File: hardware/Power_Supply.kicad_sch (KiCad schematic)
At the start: 66 parts, among them IC1 LM13700, IC2 LM13700, IC3 LM13700, J5 USB_B, SW1 POWER, U1 TL064, U19 TL064, U20 ADUM3160

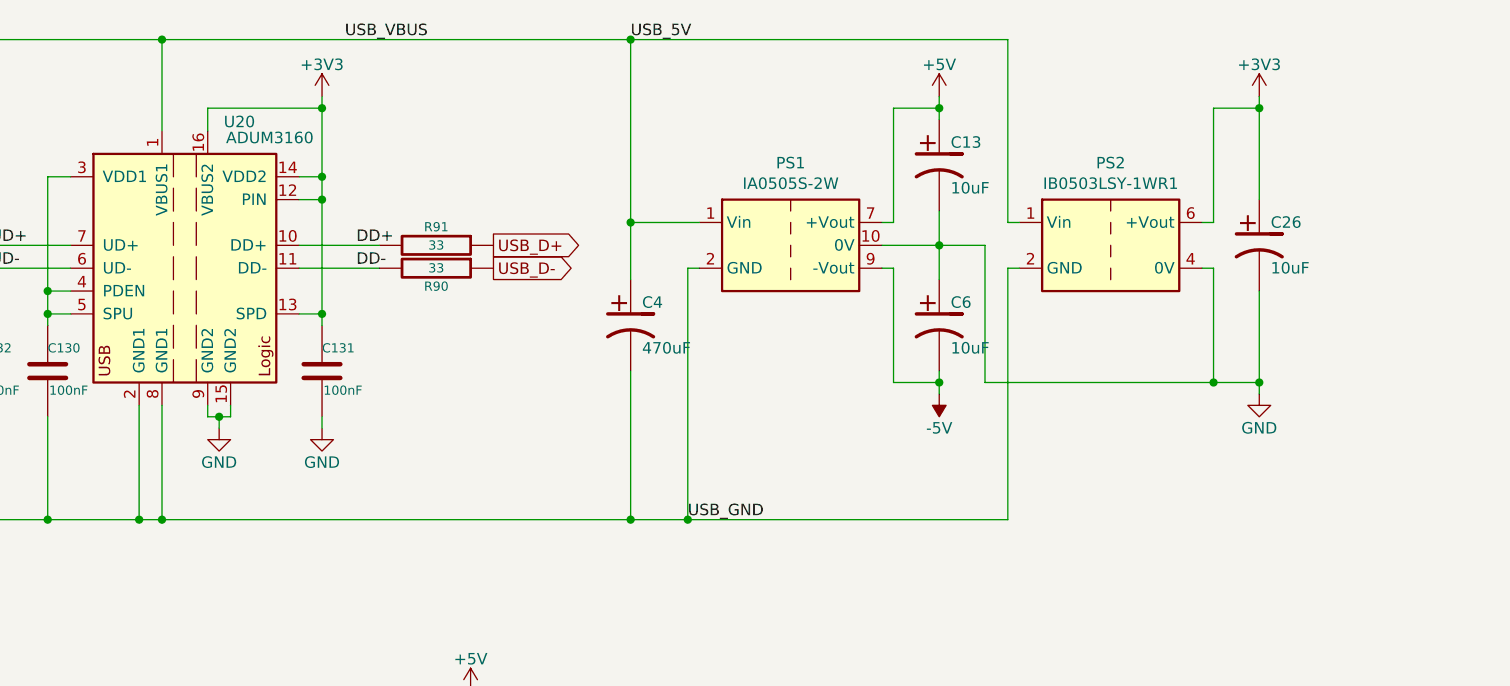
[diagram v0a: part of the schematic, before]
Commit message: hardware: add missing D+ pullup resistor (MCU side)
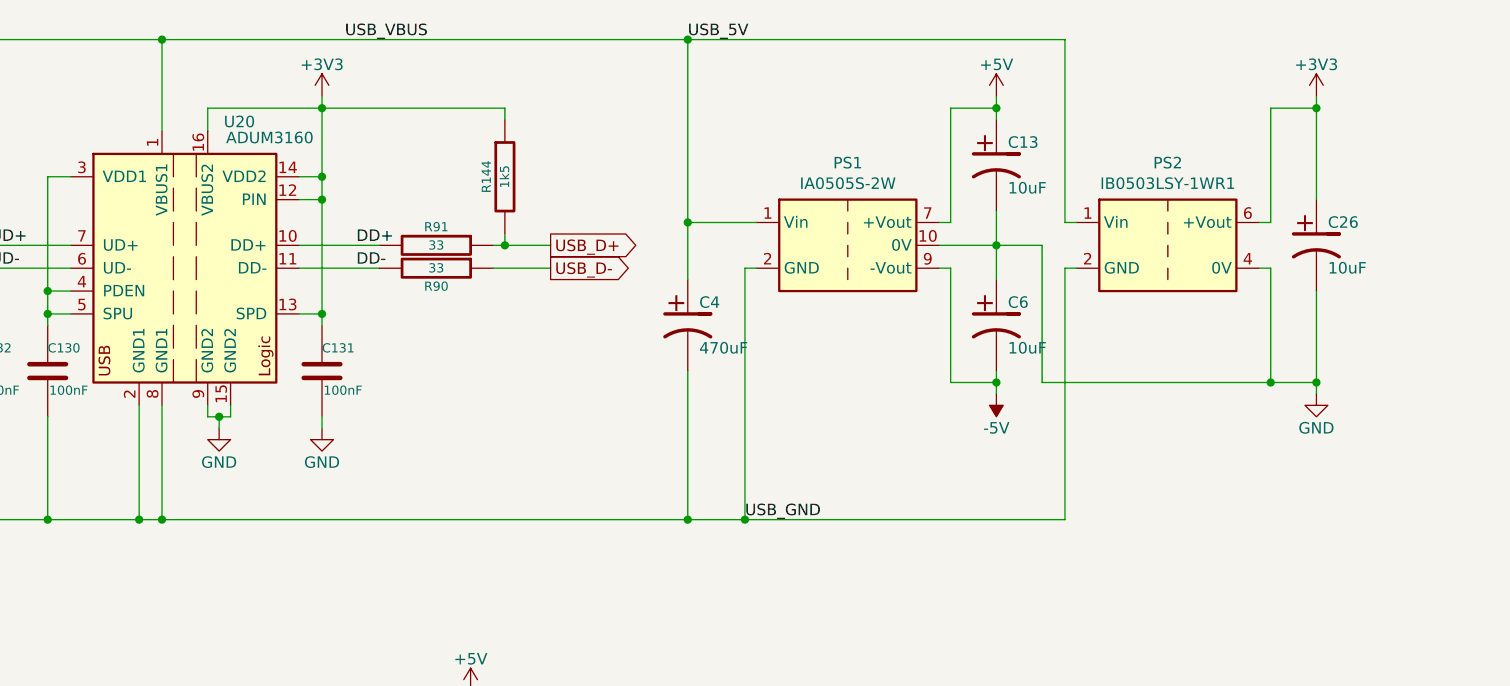
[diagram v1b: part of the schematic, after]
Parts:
- added R144: 1k5, Resistor_SMD:R_0603_1608Metric, symbol Additional:R
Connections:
- net +3V3: now also R144.1
- net USB_D+: now also R144.2
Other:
- moved on the sheet: C13, C26, C4, C6, PS1, PS2

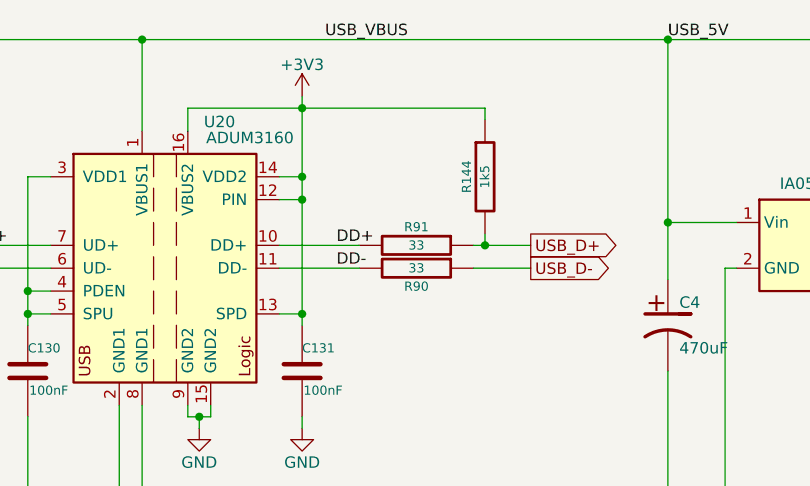
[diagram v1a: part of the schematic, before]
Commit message: Add USB pullup resistor
- Add USB pullup resistor
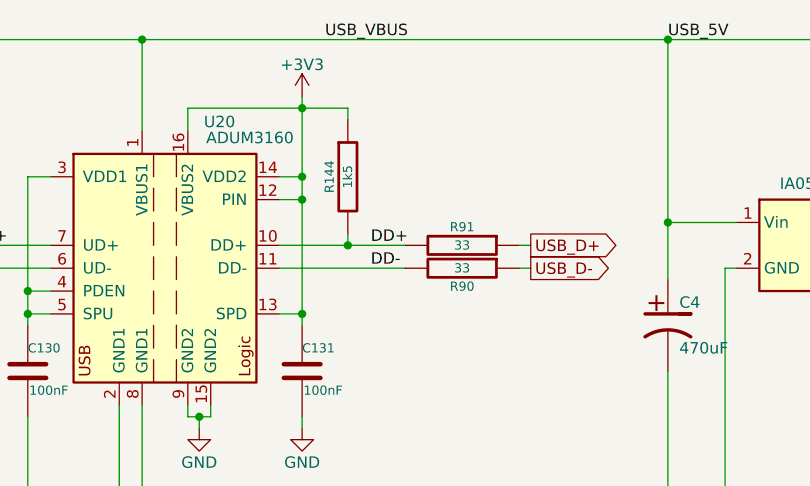
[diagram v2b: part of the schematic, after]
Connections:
- net DD+: now also R144.2
- net USB_D+: no longer R144.2
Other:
- moved on the sheet: R144, R90, R91
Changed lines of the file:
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@@
 	)
 	(junction
+		(at 137.16 55.88)
+		(diameter 0)
+		(color 0 0 0 0)
+	)
+	(junction
 		(at 106.68 125.73)
 		(diameter 0)
@@
 	)
 	(junction
-		(at 152.4 55.88)
-		(diameter 0)
-		(color 0 0 0 0)
-	)
-	(junction
 		(at 180.34 119.38)
 		(diameter 0)
@@
 	(wire
 		(pts
+			(xy 137.16 55.88) (xy 143.51 55.88)
+		)
+		(stroke
+			(width 0)
+			(type default)
+		)
+	)
+	(wire
+		(pts
 			(xy 186.69 106.68) (xy 186.69 107.95)
 		)
@@
 	(wire
 		(pts
-			(xy 152.4 55.88) (xy 151.13 55.88)
-		)
-		(stroke
-			(width 0)
-			(type default)
-		)
-	)
-	(wire
-		(pts
 			(xy 212.09 119.38) (xy 218.44 119.38)
 		)
@@
 	(wire
 		(pts
-			(xy 157.48 58.42) (xy 151.13 58.42)
+			(xy 157.48 58.42) (xy 156.21 58.42)
 		)
 		(stroke
@@
 	(wire
 		(pts
-			(xy 157.48 55.88) (xy 152.4 55.88)
+			(xy 157.48 55.88) (xy 156.21 55.88)
 		)
 		(stroke
@@
 	(wire
 		(pts
+			(xy 137.16 54.61) (xy 137.16 55.88)
+		)
+		(stroke
+			(width 0)
+			(type default)
+		)
+	)
+	(wire
+		(pts
 			(xy 132.08 40.64) (xy 132.08 48.26)
 		)
@@
 	(wire
 		(pts
-			(xy 152.4 40.64) (xy 152.4 41.91)
+			(xy 137.16 40.64) (xy 137.16 41.91)
 		)
 		(stroke
@@
 	(wire
 		(pts
-			(xy 129.54 55.88) (xy 138.43 55.88)
+			(xy 129.54 55.88) (xy 137.16 55.88)
 		)
 		(stroke
@@
 	(wire
 		(pts
-			(xy 132.08 40.64) (xy 152.4 40.64)
+			(xy 132.08 40.64) (xy 137.16 40.64)
 		)
 		(stroke
@@
 	(wire
 		(pts
-			(xy 152.4 54.61) (xy 152.4 55.88)
-		)
-		(stroke
-			(width 0)
-			(type default)
-		)
-	)
-	(wire
-		(pts
 			(xy 101.6 48.26) (xy 101.6 60.96)
 		)
@@
 	(wire
 		(pts
-			(xy 129.54 58.42) (xy 138.43 58.42)
+			(xy 129.54 58.42) (xy 143.51 58.42)
 		)
 		(stroke
@@
 	)
 	(label "DD-"
-		(at 135.89 58.42 0)
+		(at 139.7 58.42 0)
 		(fields_autoplaced yes)
 		(effects
@@
 	)
 	(label "DD+"
-		(at 135.89 55.88 0)
+		(at 139.7 55.88 0)
 		(fields_autoplaced yes)
 		(effects
@@
 	(symbol
 		(lib_id "Additional:R")
-		(at 144.78 58.42 270)
+		(at 149.86 58.42 270)
 		(unit 1)
 		(exclude_from_sim no)
@@
 		(dnp no)
 		(property "Reference" "R90"
-			(at 144.78 60.452 90)
+			(at 149.86 60.452 90)
 			(effects
 				(font
@@
 		)
 		(property "Value" "33"
-			(at 144.78 58.42 90)
+			(at 149.86 58.42 90)
 			(effects
 				(font
@@
 		)
 		(property "Footprint" "Resistor_SMD:R_0603_1608Metric"
-			(at 144.78 56.642 90)
+			(at 149.86 56.642 90)
 			(effects
 				(font
@@
 		)
 		(property "Datasheet" "~"
-			(at 144.78 58.42 0)
+			(at 149.86 58.42 0)
 			(effects
 				(font
@@
 		)
 		(property "Description" ""
-			(at 144.78 58.42 0)
+			(at 149.86 58.42 0)
 			(effects
 				(font
@@
 		)
 		(property "LCSC" "C23140"
-			(at 144.78 60.452 0)
+			(at 149.86 60.452 0)
 			(effects
 				(font
@@
 	(symbol
 		(lib_id "Additional:R")
-		(at 152.4 48.26 0)
+		(at 137.16 48.26 0)
 		(unit 1)
 		(exclude_from_sim no)
@@
 		(dnp no)
 		(property "Reference" "R144"
-			(at 150.368 48.26 90)
+			(at 135.128 48.26 90)
 			(effects
 				(font
@@
 		)
 		(property "Value" "1k5"
-			(at 152.4 48.26 90)
+			(at 137.16 48.26 90)
 			(effects
 				(font
@@
 		)
 		(property "Footprint" "Resistor_SMD:R_0603_1608Metric"
-			(at 150.622 48.26 90)
+			(at 135.382 48.26 90)
 			(effects
 				(font
@@
 		)
 		(property "Datasheet" "~"
-			(at 152.4 48.26 0)
+			(at 137.16 48.26 0)
 			(effects
 				(font
@@
 		)
 		(property "Description" ""
-			(at 152.4 48.26 0)
+			(at 137.16 48.26 0)
 			(effects
 				(font
@@
 		)
 		(property "LCSC" "C22843"
-			(at 154.432 48.26 0)
+			(at 139.192 48.26 0)
 			(effects
 				(font
@@
 	(symbol
 		(lib_id "Additional:R")
-		(at 144.78 55.88 270)
+		(at 149.86 55.88 270)
 		(unit 1)
 		(exclude_from_sim no)
@@
 		(dnp no)
 		(property "Reference" "R91"
-			(at 144.78 53.848 90)
+			(at 149.86 53.848 90)
 			(effects
 				(font
@@
 		)
 		(property "Value" "33"
-			(at 144.78 55.88 90)
+			(at 149.86 55.88 90)
 			(effects
 				(font
@@
 		)
 		(property "Footprint" "Resistor_SMD:R_0603_1608Metric"
-			(at 144.78 54.102 90)
+			(at 149.86 54.102 90)
 			(effects
 				(font
@@
 		)
 		(property "Datasheet" "~"
-			(at 144.78 55.88 0)
+			(at 149.86 55.88 0)
 			(effects
 				(font
@@
 		)
 		(property "Description" ""
-			(at 144.78 55.88 0)
+			(at 149.86 55.88 0)
 			(effects
 				(font
@@
 		)
 		(property "LCSC" "C23140"
-			(at 144.78 57.912 0)
+			(at 149.86 57.912 0)
 			(effects
 				(font

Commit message: hardware: updated some LCSC references
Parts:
- U20: LCSC C284149 -> C284149
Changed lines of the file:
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@@
 			)
 		)
-		(property "LCSC" " C284149"
+		(property "LCSC" "C284149"
 			(at 116.84 58.42 0)
 			(effects
